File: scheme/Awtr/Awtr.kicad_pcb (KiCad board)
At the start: 2 copper layers, 45.4 x 30.3 mm, 12 parts, among them J1 Barrel_Jack_Switch, J2 WCH_Link, J3 Water_pump, J4 Sensor, Q1 IRLB8743, SW1 SW_Push, U1 CH32V003J4M6

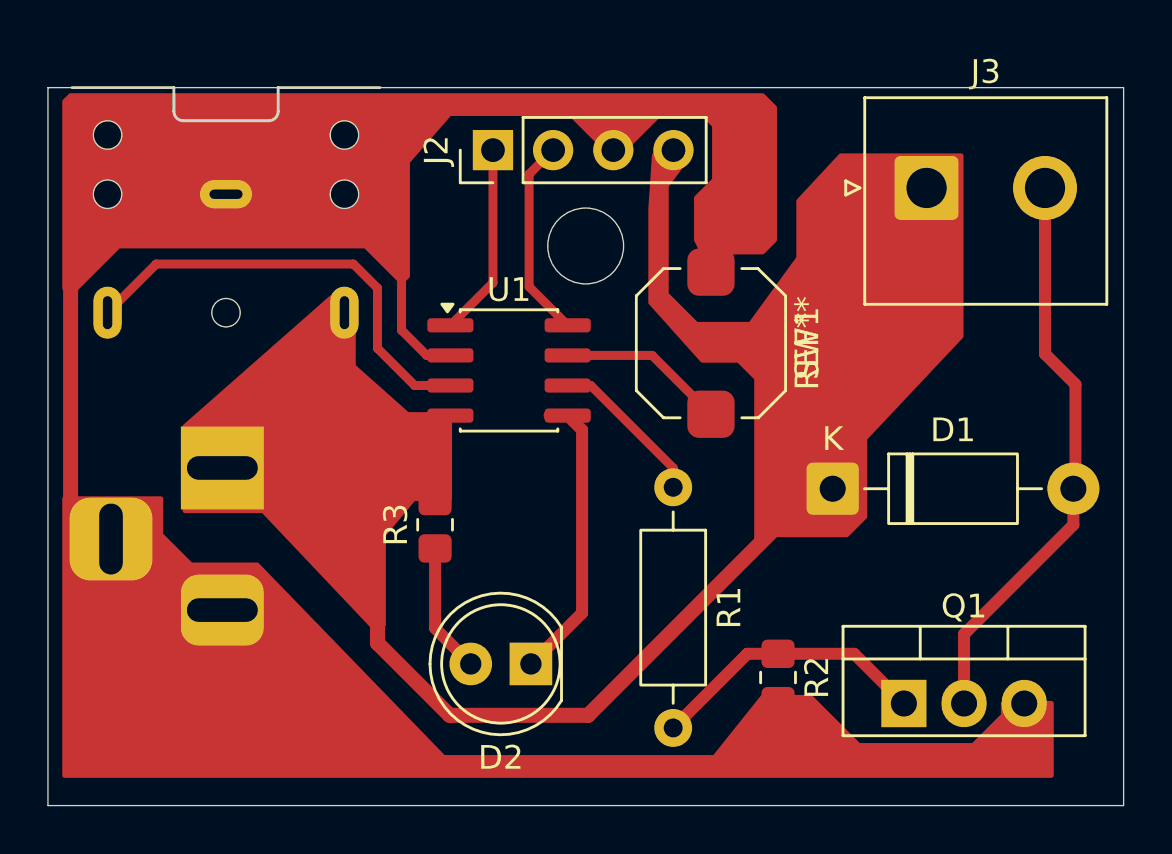
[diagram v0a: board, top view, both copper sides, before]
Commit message: +ADC
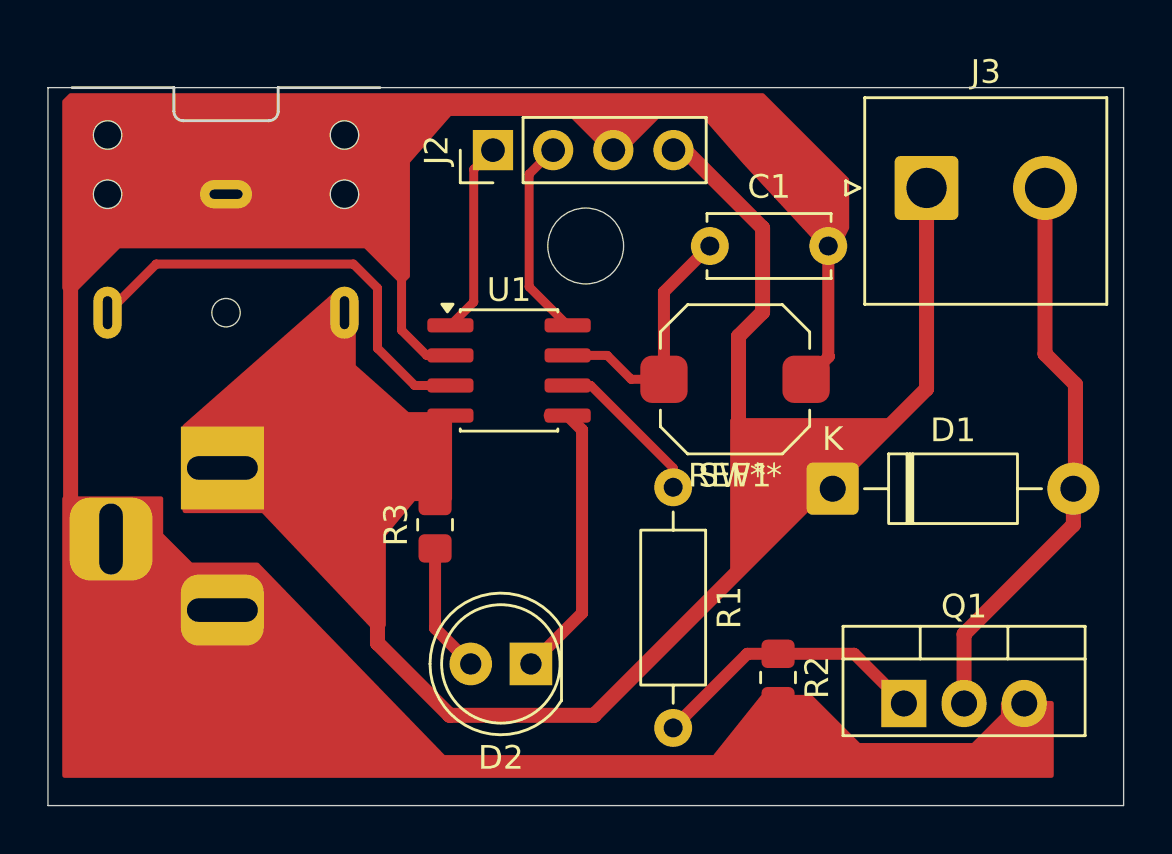
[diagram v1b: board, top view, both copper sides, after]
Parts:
- added C1: 10pF, Capacitor_THT:C_Disc_D5.0mm_W2.5mm_P5.00mm, F.Cu at (106.5, 40.1)
- moved SW1 1.83 mm to (107.5, 45.8), turned to 180 degrees
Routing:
- net +5V: track 47.8 -> 68.7 mm
- net Net-(U1-PC4): track 7.08 -> 10.9 mm
- net GND: track 67.6 -> 65.8 mm
